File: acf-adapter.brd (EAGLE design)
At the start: 98.4 x 49.5 mm, 87 parts, among them IC1 UCC27712, IC2 UCC28780, IC3 TL431, Q1 2SK3115, Q2 TK13A60, Q3 2N7002, Q4 BSS127, Q5 TLP621-1, T1 COMMON_FILTER-SU10VFC, T2 TRANSFORMAER_FLYBACK-PQ2620-A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

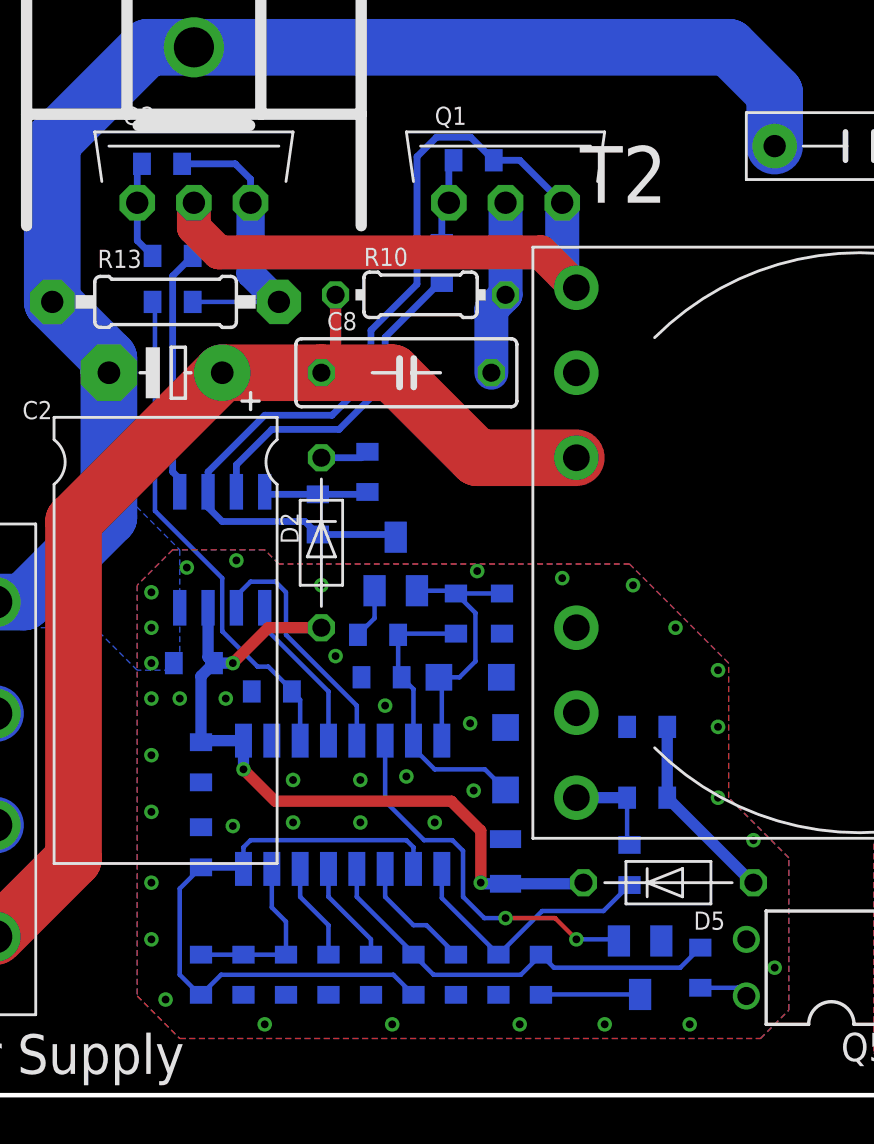
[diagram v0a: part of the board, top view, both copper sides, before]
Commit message: 発注
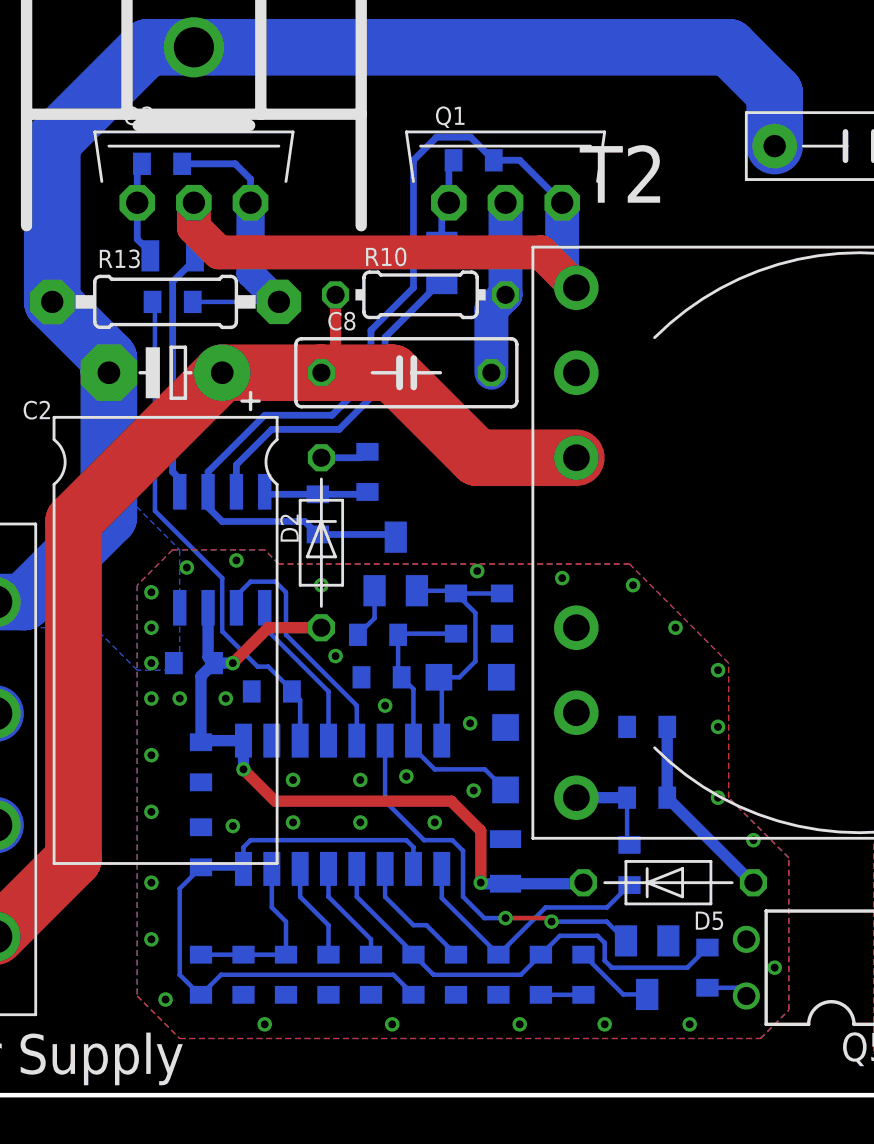
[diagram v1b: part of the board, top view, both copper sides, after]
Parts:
- added R30: 240k, my_rcl:1608
- R1: value 250k -> 240k
- R14: value 1M -> 240k
- R15: value 470k -> 240k
- R2: value 125k -> 120k
- R27: value 10 -> 120
- R8, R9: device my_rcl:1608 -> my_rcl:2012
- moved Q3 0.32 mm to (48.9, 5.71)
- moved R17 0.32 mm to (51.6, 5.71)
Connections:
- new net N$37: R15.1, R30.1
- net N$34: now also R30.2; no longer R15.1
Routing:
- net N$37: track 0.00 -> 1.91 mm
- net FB: track 19.1 -> 20.6 mm
- net N$34: track 4.45 -> 3.60 mm
